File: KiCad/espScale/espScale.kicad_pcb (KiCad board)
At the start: 2 copper layers, 46.4 x 71.1 mm, 1 part, among them U1 NodeMCU1.0(ESP-12E)

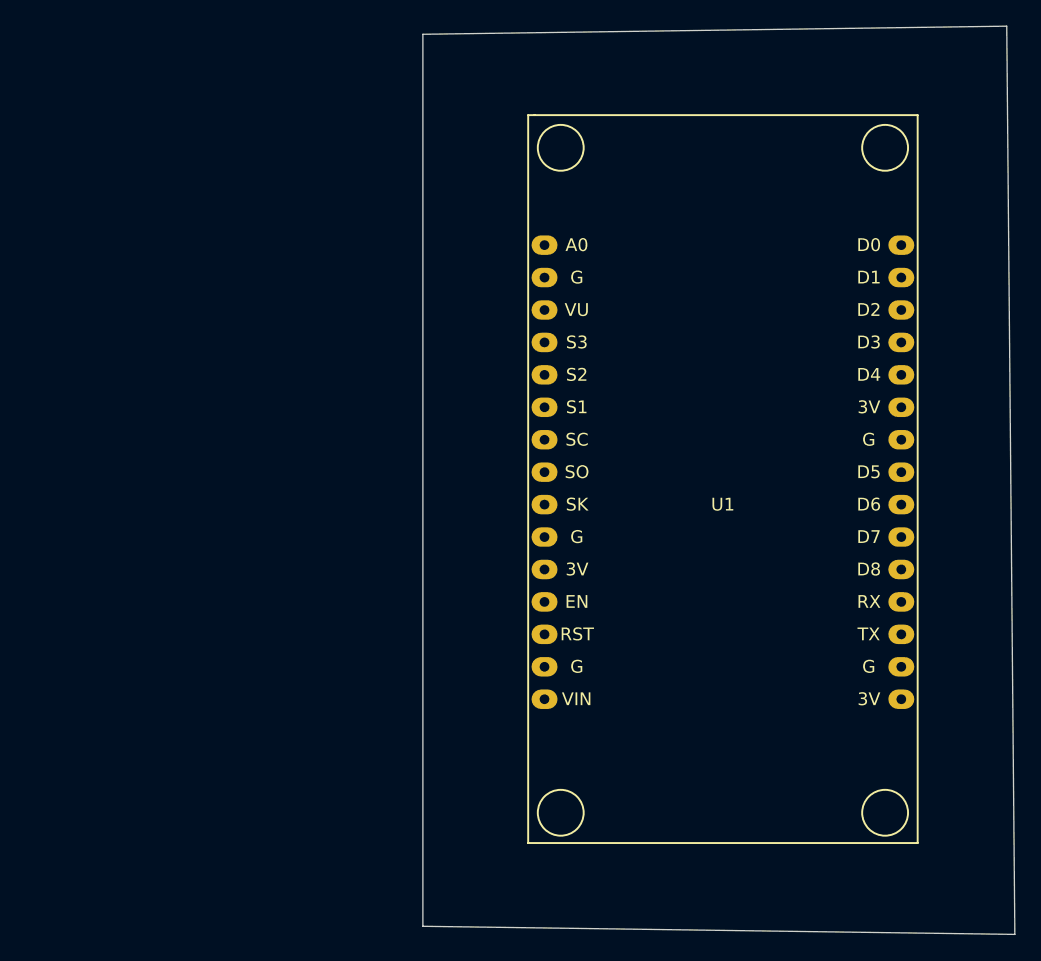
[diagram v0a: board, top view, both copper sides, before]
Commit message: pcb
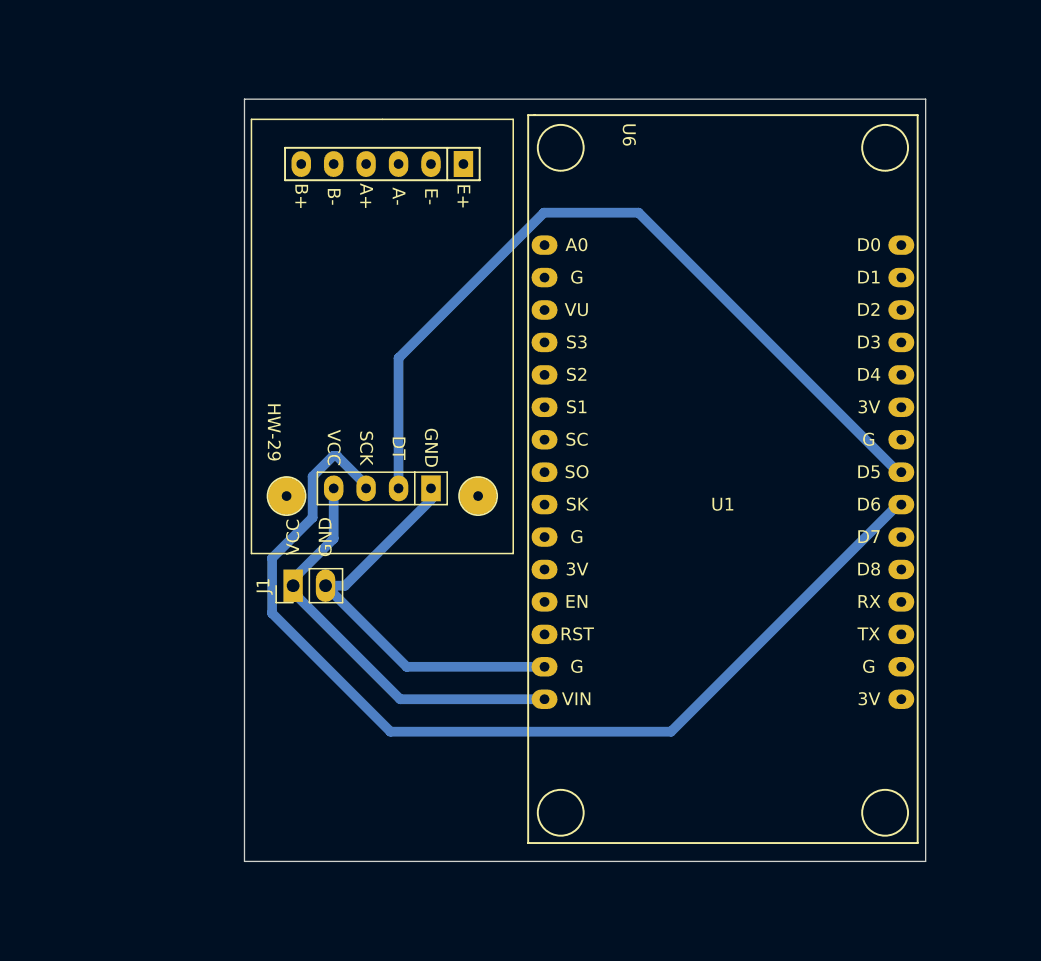
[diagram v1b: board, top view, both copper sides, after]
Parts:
- added J1: 2-pin_power_input_header, My_Headers:2-pin_power_input_header_larger_pads, F.Cu at (108.0, 101.6)
- added U6: HX711_Load_Cell_Amplifier, My_Parts:HX711 Load Cell Amplifier w_pinsockets_large, F.Cu at (114.9, 68.6)
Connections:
- U1 pad 22: unconnected-(U1-Pad22) -> SCK
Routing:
- net SCK: track 0.00 -> 78.6 mm
- net DT: track 0.00 -> 62.7 mm
- net +5V: track 0.00 -> 32.6 mm
- net GND: track 0.00 -> 31.7 mm
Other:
- board size 46.4 x 71.1 mm -> 53.3 x 59.7 mm

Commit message: kicad
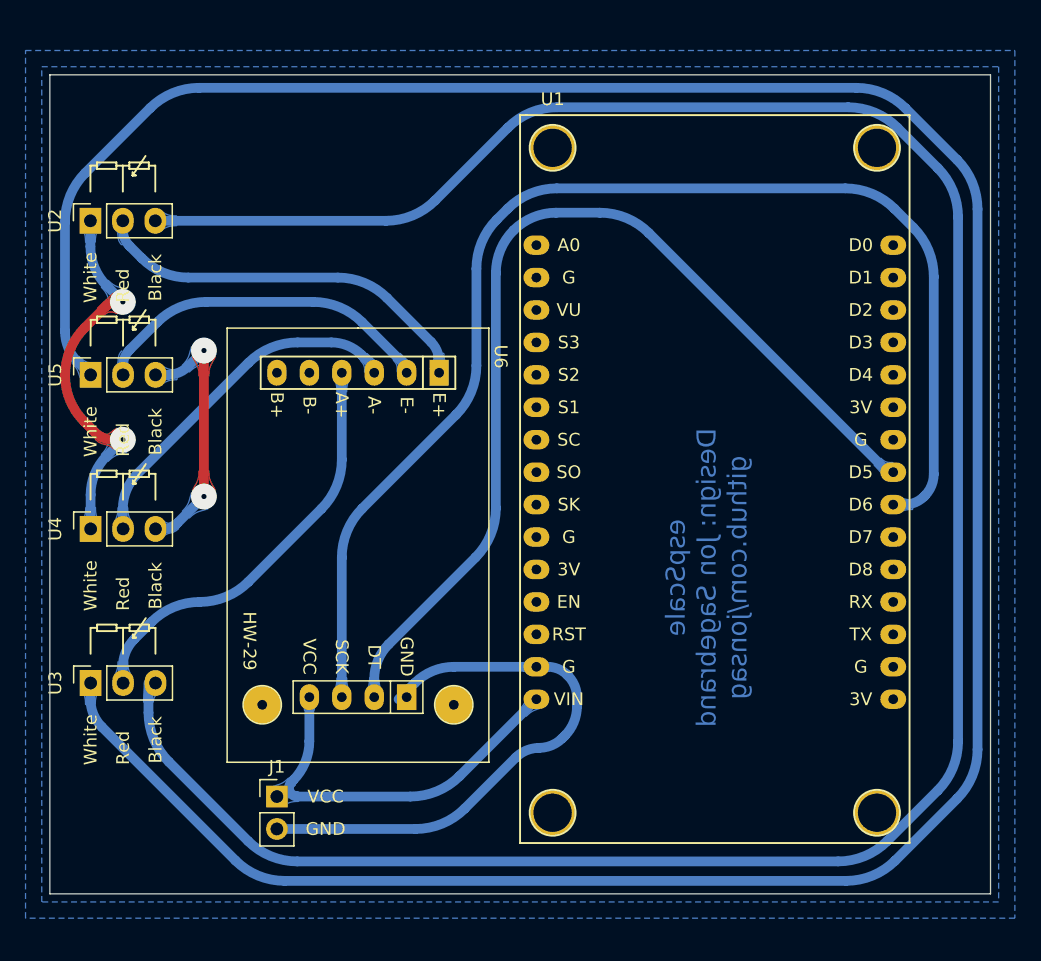
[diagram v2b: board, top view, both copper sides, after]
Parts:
- added U2: 3-wire_Load_Cell, My_Headers:3-pin_load_cell_header_large, F.Cu at (92.1, 73.0)
- added U3: ~, My_Headers:3-pin_load_cell_header_large, F.Cu at (92.1, 109.2)
- added U4: 3-wire_Load_Cell, My_Headers:3-pin_load_cell_header_large, F.Cu at (92.1, 97.2)
- added U5: ~, My_Headers:3-pin_load_cell_header_large, F.Cu at (92.1, 85.1)
- J1: footprint My_Headers:2-pin_power_input_header_larger_pads -> My_Headers:2-pin_power_input_header
- moved U1 25.0 mm to (127.0, 74.9)
- moved U6 16.9 mm to (119.4, 84.9)
- moved J1 16.6 mm to (106.7, 118.1), turned to 0 degrees
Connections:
- U6 pad 3: (no net) -> Net-(U6-Pad3)
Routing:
- net Net-(U3-Pad1): track 0.00 -> 218.3 mm
- net Net-(U2-Pad3): track 0.00 -> 187.5 mm
- net Net-(U3-Pad2): track 0.00 -> 33.1 mm
- net Net-(U2-Pad2): track 0.00 -> 30.9 mm
- net Net-(U2-Pad1): track 0.00 -> 30.4 mm, vias 0 -> 2
- net Net-(U6-Pad3): track 0.00 -> 28.2 mm
- net Net-(U5-Pad2): track 0.00 -> 26.9 mm
- net SCK: track 78.6 -> 100.2 mm
- net Net-(U4-Pad3): track 0.00 -> 20.7 mm, vias 0 -> 2
- net DT: track 62.7 -> 78.8 mm
- net GND: track 31.7 -> 44.5 mm
- net +5V: track 32.6 -> 30.6 mm
- added copper zone on B.Cu, net (none)
- added copper zone on B.Cu, net GND
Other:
- board size 53.3 x 59.7 mm -> 73.7 x 64.1 mm
- board text added: "espScale Design: Jon Sagebrand github.com/jonsag"
